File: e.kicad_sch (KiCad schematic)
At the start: 10 parts, among them SW1 usr, SW2 rst, U1 Display_ST7789, U2 MAX98357A

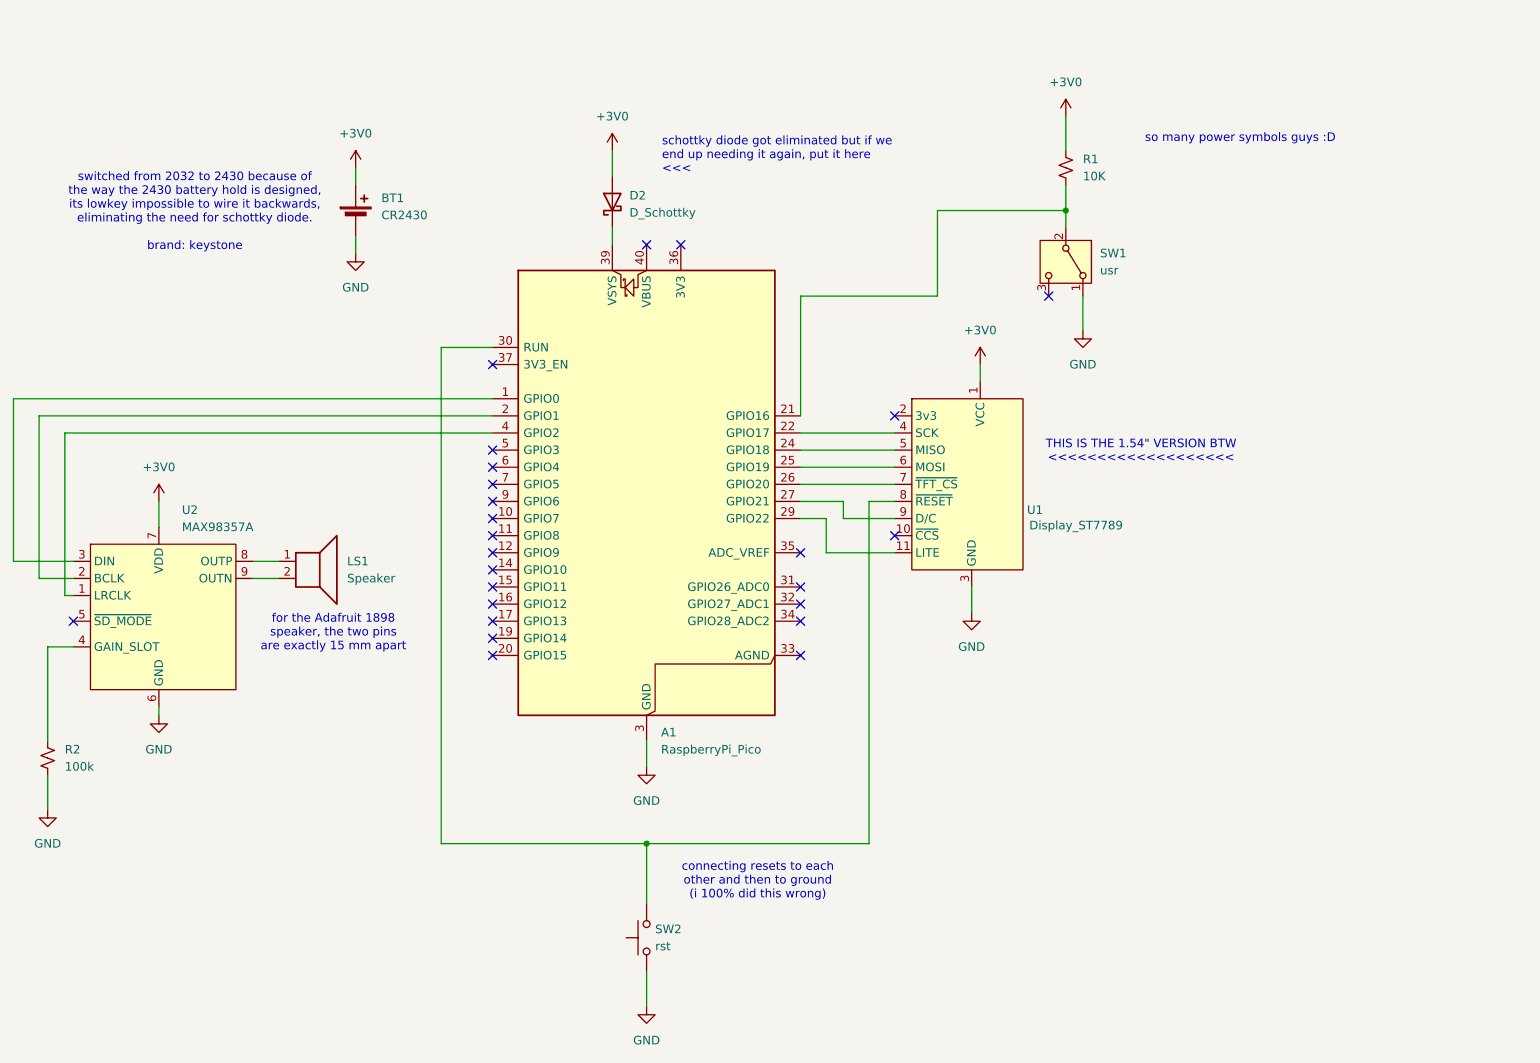
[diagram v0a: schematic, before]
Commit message: fixed so many things (i hope)
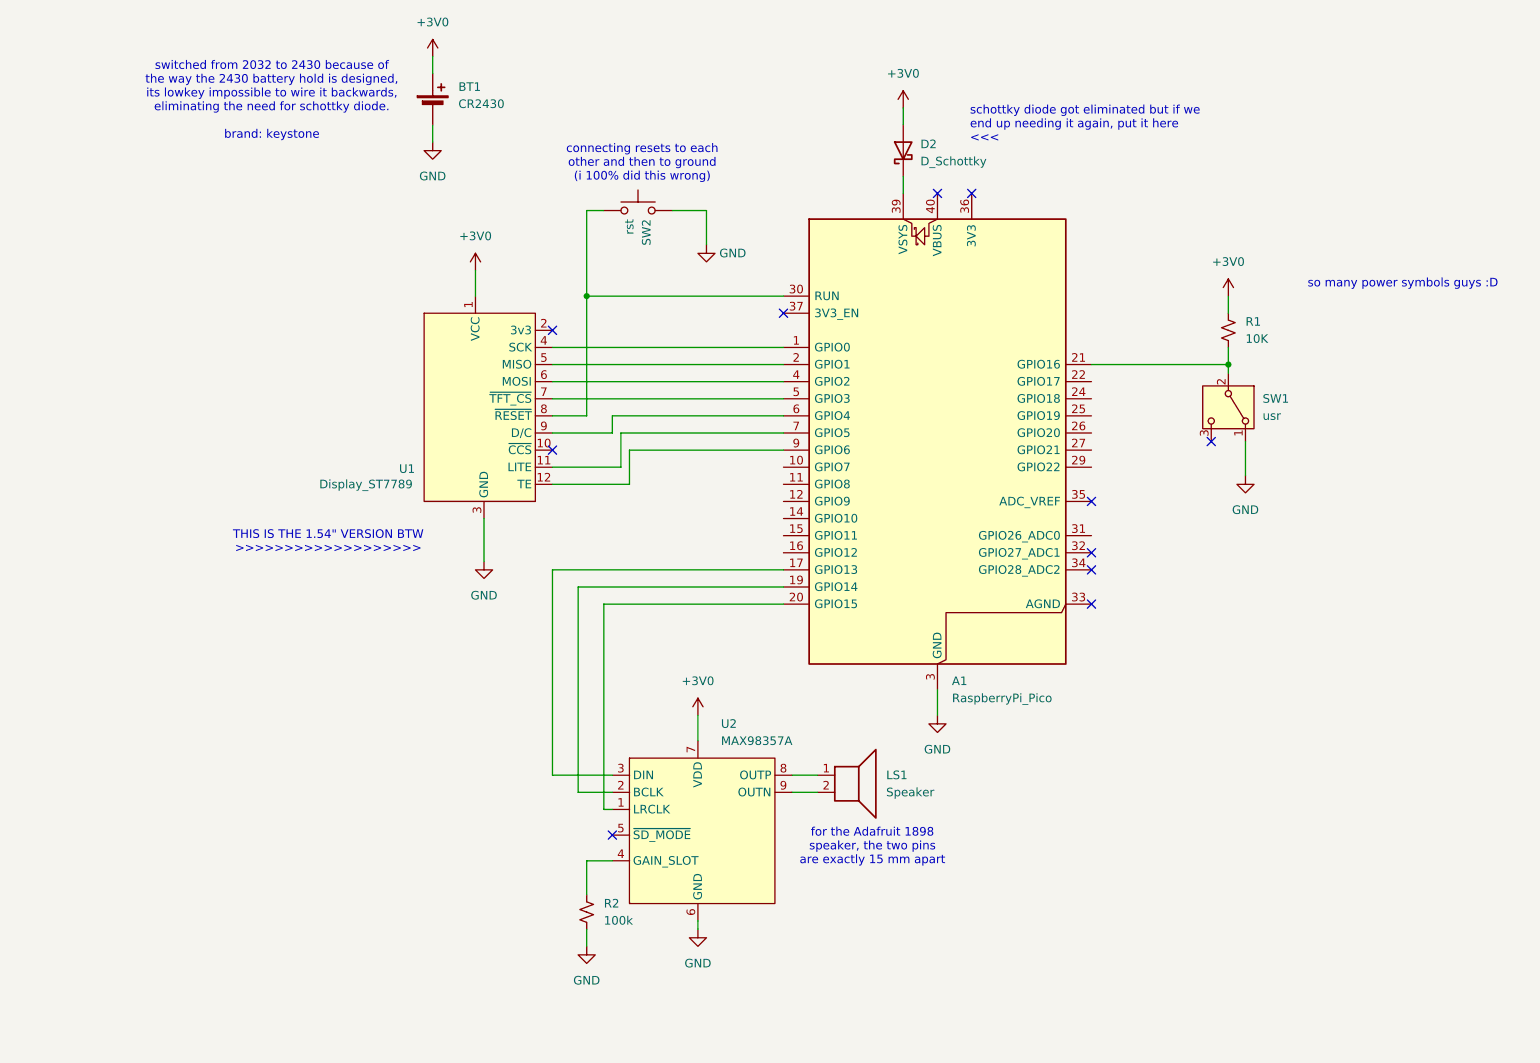
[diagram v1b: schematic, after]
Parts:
- U2: footprint MAX98357A:MAX98357A -> amp-of-doom:MAX98357A
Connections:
- net GND: now also SW2.2; no longer SW2.1
- net at U2.1 (LRCLK): now also A1.20 (GPIO15); no longer A1.4 (GPIO2)
- net at U2.2 (BCLK): now also A1.19 (GPIO14); no longer A1.2 (GPIO1)
- net at U2.3 (DIN): now also A1.17 (GPIO13); no longer A1.1 (GPIO0)
- net at U1.4 (SCK): now also A1.1 (GPIO0); no longer A1.22 (GPIO17)
- net at U1.5 (MISO): now also A1.2 (GPIO1); no longer A1.24 (GPIO18)
- net at A1.25 (GPIO19): no longer U1.6 (MOSI)
- net at A1.26 (GPIO20): no longer U1.7 (~{TFT_CS})
- net at A1.27 (GPIO21): no longer U1.9 (D/C)
- net at A1.29 (GPIO22): no longer U1.11 (LITE)
- net at A1.30 (RUN), U1.8 (~{RESET}): now also SW2.1; no longer SW2.2
- net at A1.5 (GPIO3): now also U1.7 (~{TFT_CS})
- net at A1.6 (GPIO4): now also U1.9 (D/C)
- net at A1.7 (GPIO5): now also U1.11 (LITE)
- net at A1.9 (GPIO6): now also U1.12 (TE)
- new net: A1.4 (GPIO2), U1.6 (MOSI)
- no-connect marks 25 -> 11
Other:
- note added: "THIS IS THE 1.54" VERSION BTW >>>>>>>>>>>>>>>>>>>"
- note removed: "THIS IS THE 1.54" VERSION BTW <<<<<<<<<<<<<<<<<<<"
- moved on the sheet: A1, BT1, D2, LS1, R1, R2, SW1, U2
